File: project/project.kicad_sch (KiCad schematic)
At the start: 26 parts, among them J1 Conn_01x03, J2 Conn_02x07_Odd_Even, J3 Conn_01x02, J5 12V, Q1 IRF4905, Q2 NPN, SW1 SW_Push, U1 module_ina219

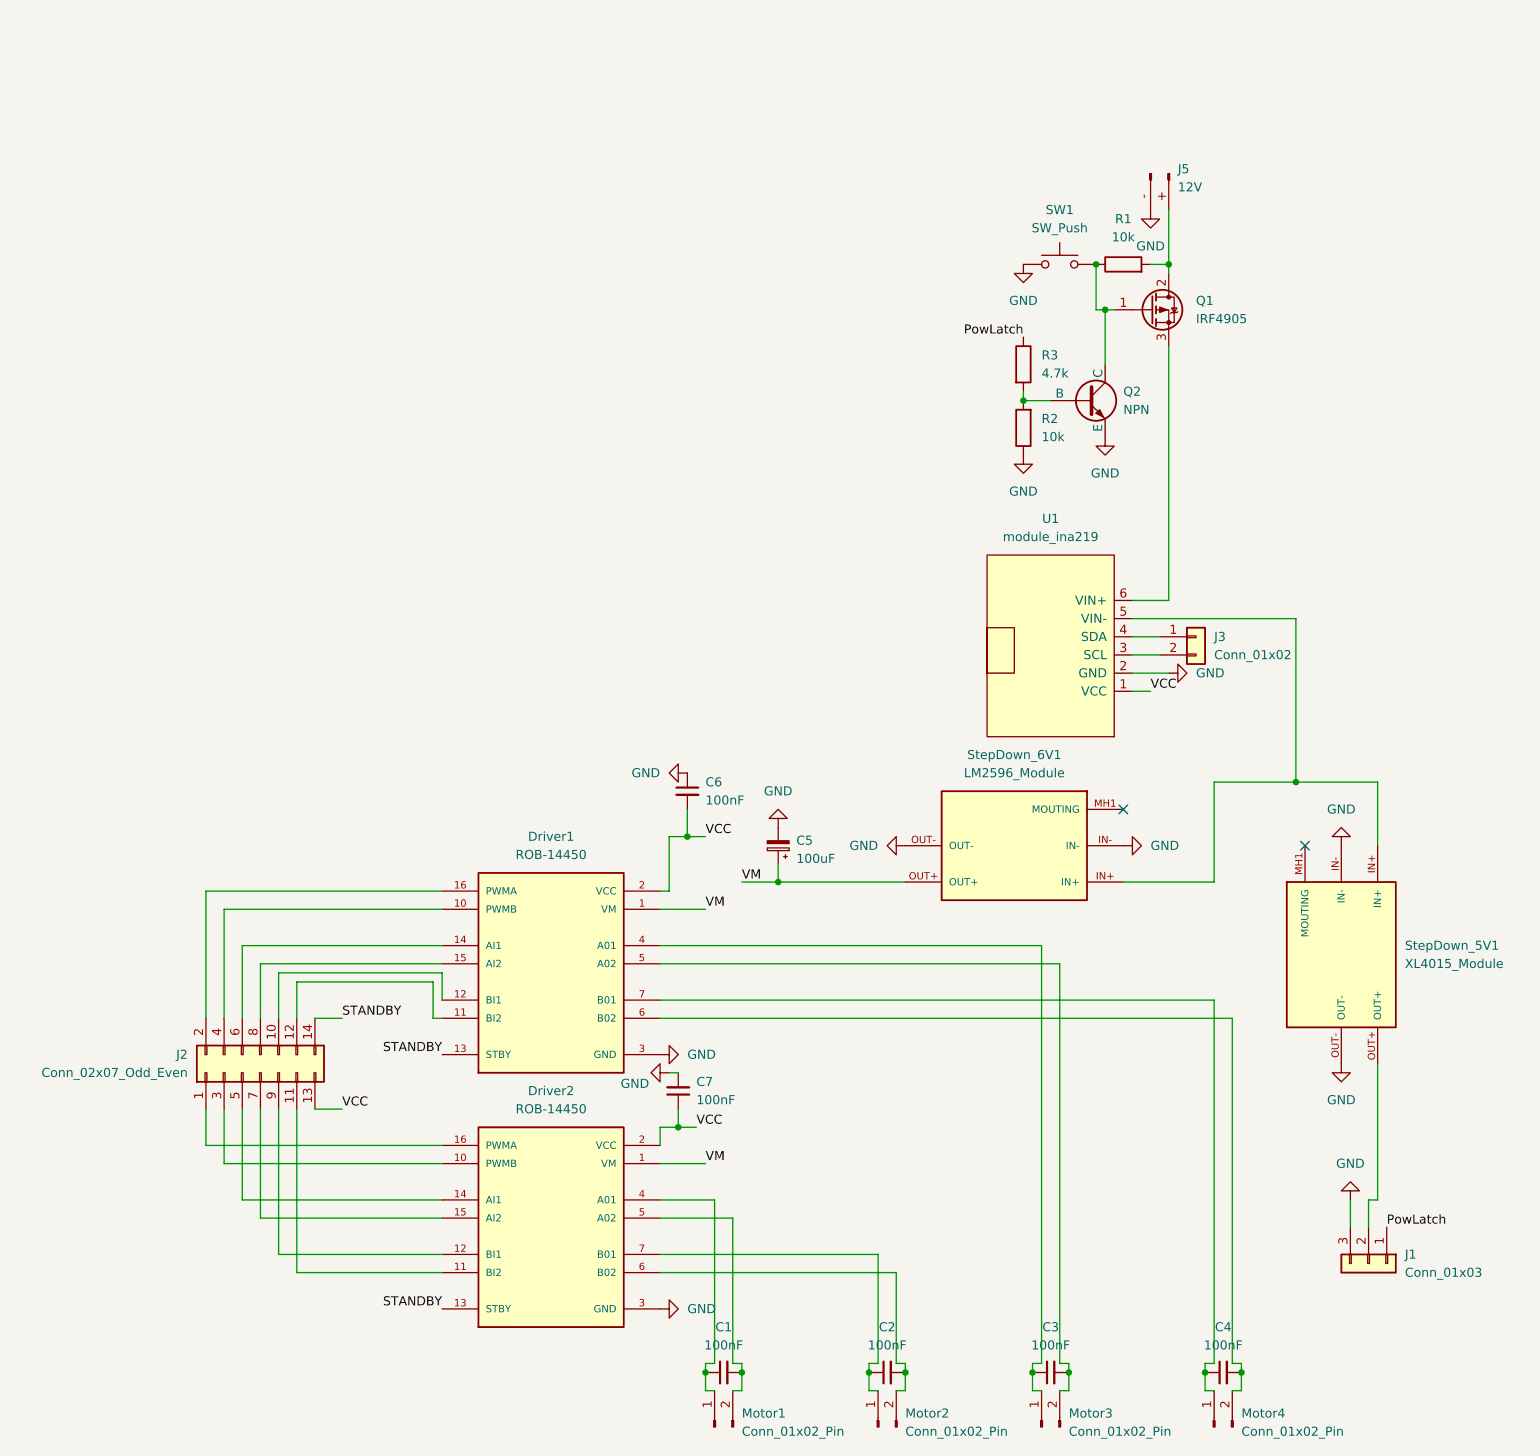
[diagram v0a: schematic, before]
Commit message: last-update
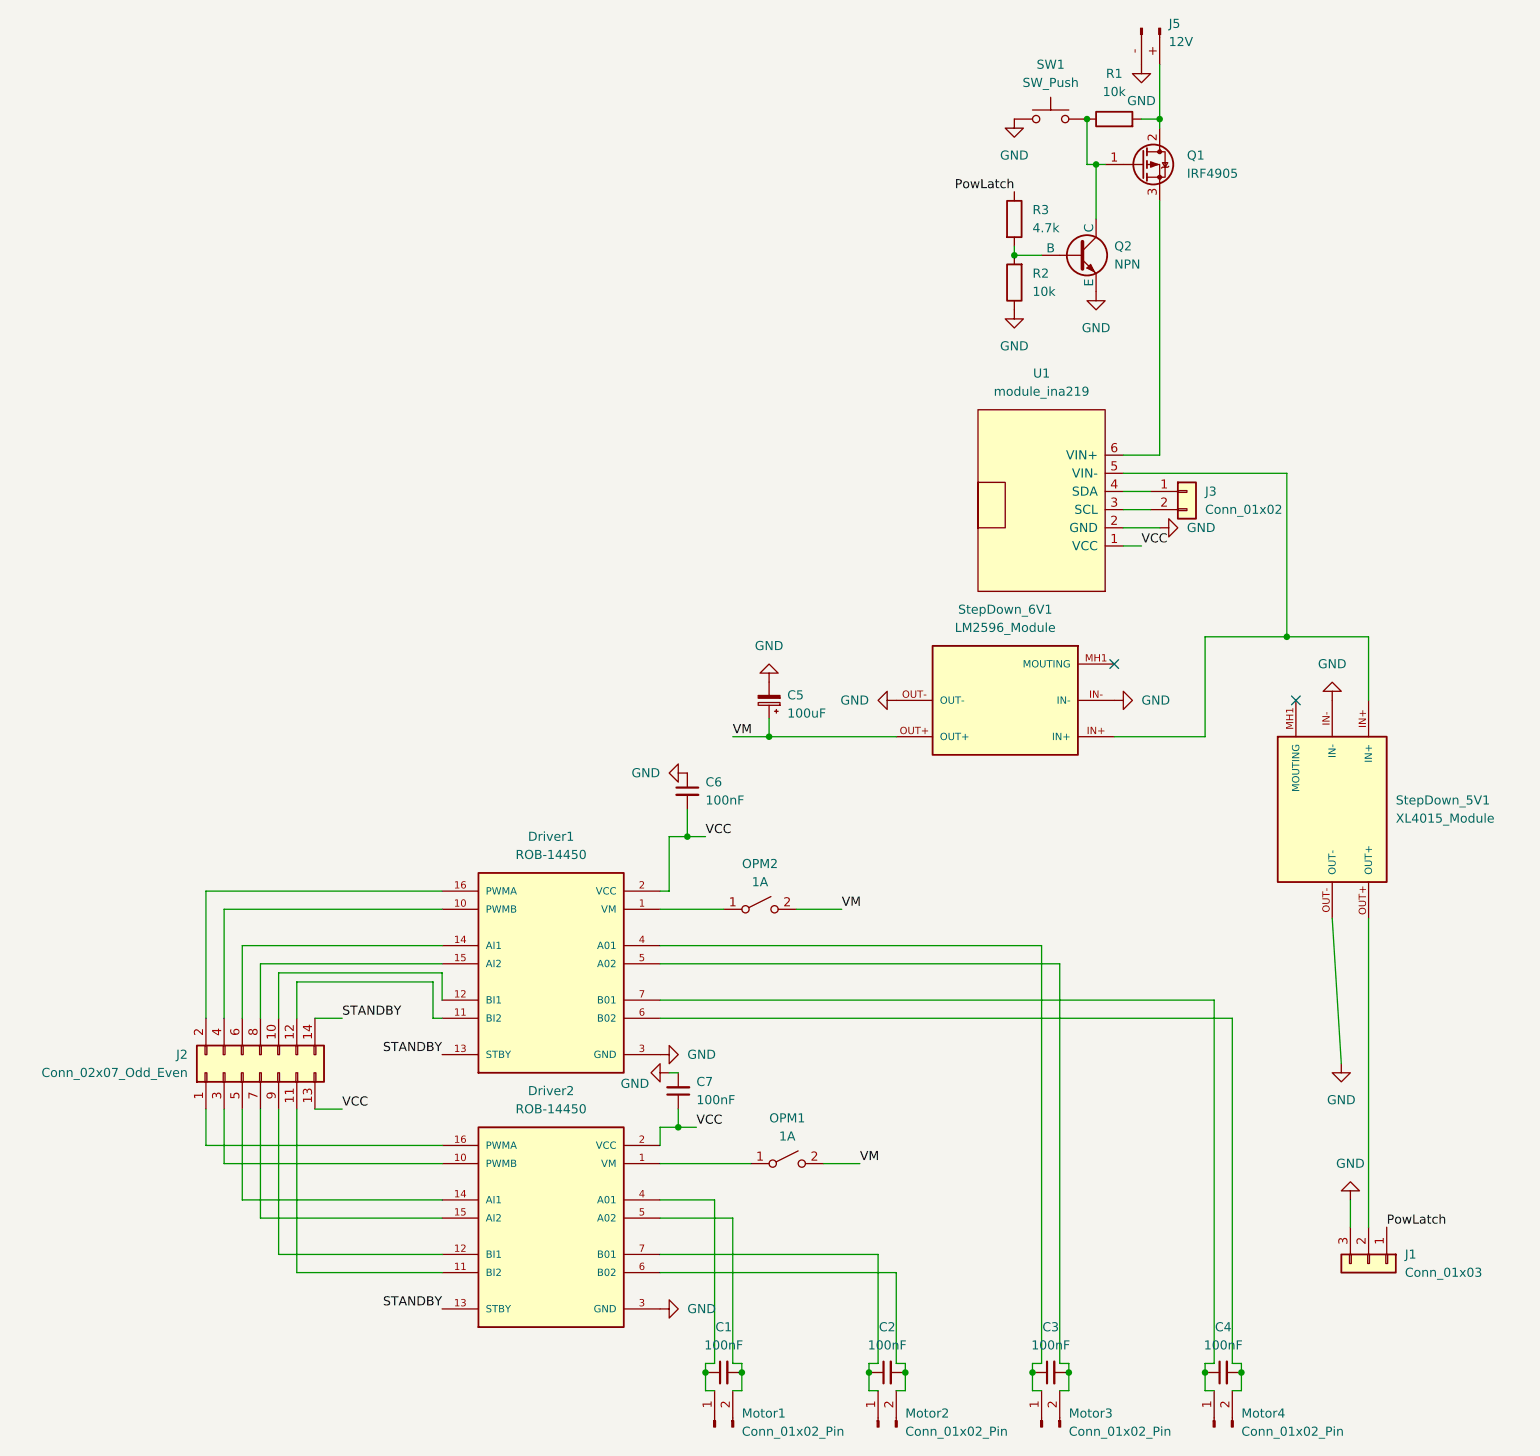
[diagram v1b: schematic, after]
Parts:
- added OPM1, OPM2: 1A, byRadu:OPM_Kuoyuh_91, symbol Switch:SW_SPST
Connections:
- net VM: now also OPM1.2 (B), OPM2.2 (B); no longer Driver1.1 (VM), Driver2.1 (VM)
- new net: Driver2.1 (VM), OPM1.1 (A)
- new net: Driver1.1 (VM), OPM2.1 (A)
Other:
- moved on the sheet: C5, J3, J5, Q1, Q2, R1, R2, R3, SW1, StepDown_5V1, StepDown_6V1, U1

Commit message: updated capacitor size
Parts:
- C1, C2, C3, C4, C6, C7: footprint Capacitor_SMD:C_0603_1608Metric_Pad1.08x0.95mm_HandSolder -> Capacitor_SMD:C_1206_3216Metric_Pad1.33x1.80mm_HandSolder
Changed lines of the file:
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@@
 			)
 		)
-		(property "Footprint" "Capacitor_SMD:C_0603_1608Metric_Pad1.08x0.95mm_HandSolder"
+		(property "Footprint" "Capacitor_SMD:C_1206_3216Metric_Pad1.33x1.80mm_HandSolder"
 			(at 189.23 250.19 0)
 			(hide yes)
@@
 			)
 		)
-		(property "Footprint" "Capacitor_SMD:C_0603_1608Metric_Pad1.08x0.95mm_HandSolder"
+		(property "Footprint" "Capacitor_SMD:C_1206_3216Metric_Pad1.33x1.80mm_HandSolder"
 			(at 213.36 250.19 0)
 			(hide yes)
@@
 			)
 		)
-		(property "Footprint" "Capacitor_SMD:C_0603_1608Metric_Pad1.08x0.95mm_HandSolder"
+		(property "Footprint" "Capacitor_SMD:C_1206_3216Metric_Pad1.33x1.80mm_HandSolder"
 			(at 166.37 250.19 0)
 			(hide yes)
@@
 			)
 		)
-		(property "Footprint" "Capacitor_SMD:C_0603_1608Metric_Pad1.08x0.95mm_HandSolder"
+		(property "Footprint" "Capacitor_SMD:C_1206_3216Metric_Pad1.33x1.80mm_HandSolder"
 			(at 138.43 168.91 0)
 			(hide yes)
@@
 			)
 		)
-		(property "Footprint" "Capacitor_SMD:C_0603_1608Metric_Pad1.08x0.95mm_HandSolder"
+		(property "Footprint" "Capacitor_SMD:C_1206_3216Metric_Pad1.33x1.80mm_HandSolder"
 			(at 137.16 210.82 0)
 			(hide yes)
@@
 			)
 		)
-		(property "Footprint" "Capacitor_SMD:C_0603_1608Metric_Pad1.08x0.95mm_HandSolder"
+		(property "Footprint" "Capacitor_SMD:C_1206_3216Metric_Pad1.33x1.80mm_HandSolder"
 			(at 143.51 250.19 0)
 			(hide yes)
